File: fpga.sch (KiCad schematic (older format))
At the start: 107 parts, among them J14 JTAG, J19 TP_NORM_Y_G, J20 TP_RGB_COMP_X, J21 TP_HD_SD_X, SW1 FORCE_VIDEO, SW2 FORCE_VIDEO, U10 74LVC541A, U12 TC7SZ125FU, U15 10M08SC, U19 74LVC2G34, U5 74LVC14A, U6 74LVC14A, U7 74LVC14A, U9 KC2520Z50

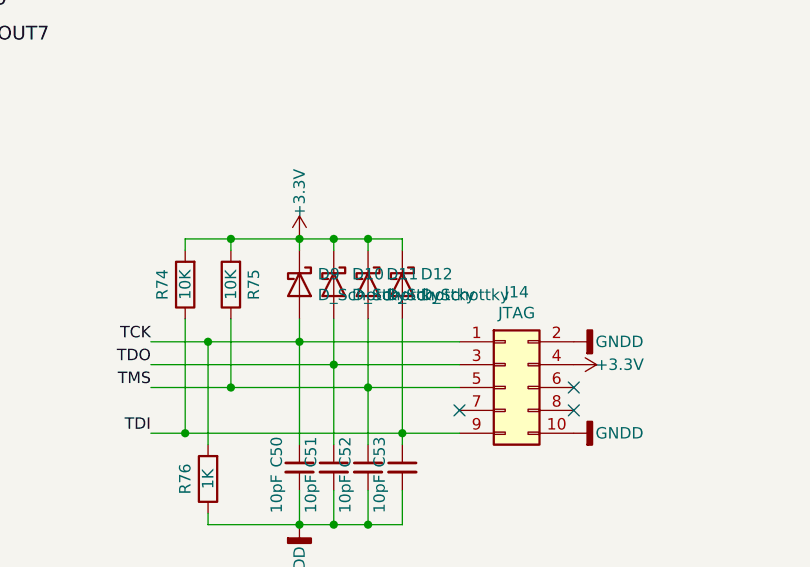
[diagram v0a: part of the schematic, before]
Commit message: Rev. E1
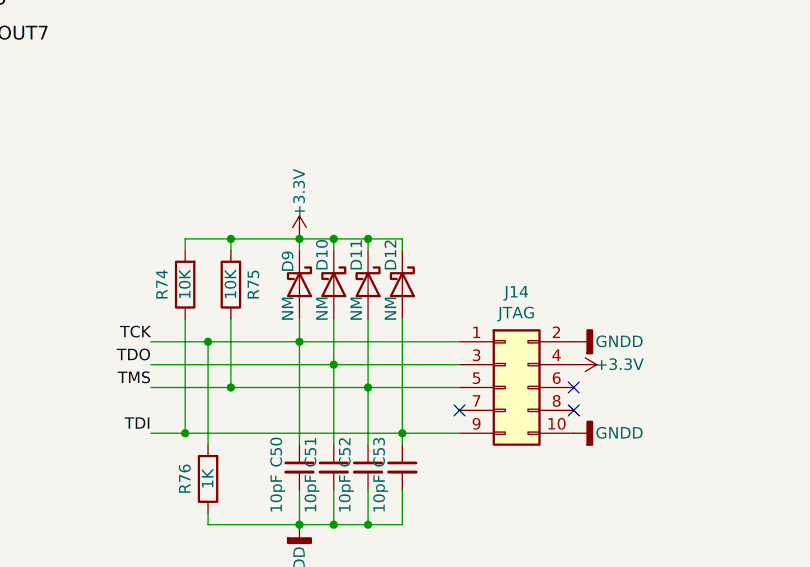
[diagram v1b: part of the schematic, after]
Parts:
- D10, D11, D12, D9: value D_Schottky -> NM
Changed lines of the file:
@@
 U 1 1 60BEE0A2
 P 8000 9450
-F 0 "D9" V 7954 9530 50  0000 L CNN
-F 1 "D_Schottky" V 8045 9530 50  0000 L CNN
+F 0 "D9" H 7850 9400 50  0000 L CNN
+F 1 "NM" H 8050 9400 50  0000 L CNN
 F 2 "Diode_SMD:D_SOD-123" H 8000 9450 50  0001 C CNN
 F 3 "~" H 8000 9450 50  0001 C CNN
@@
 U 1 1 60BFCE92
 P 8150 9450
-F 0 "D10" V 8104 9530 50  0000 L CNN
-F 1 "D_Schottky" V 8195 9530 50  0000 L CNN
+F 0 "D10" H 7950 9400 50  0000 L CNN
+F 1 "NM" H 8200 9400 50  0000 L CNN
 F 2 "Diode_SMD:D_SOD-123" H 8150 9450 50  0001 C CNN
 F 3 "~" H 8150 9450 50  0001 C CNN
@@
 U 1 1 60BFDBA6
 P 8300 9450
-F 0 "D11" V 8254 9530 50  0000 L CNN
-F 1 "D_Schottky" V 8345 9530 50  0000 L CNN
+F 0 "D11" H 8100 9400 50  0000 L CNN
+F 1 "NM" H 8350 9400 50  0000 L CNN
 F 2 "Diode_SMD:D_SOD-123" H 8300 9450 50  0001 C CNN
 F 3 "~" H 8300 9450 50  0001 C CNN
@@
 U 1 1 60BFE268
 P 8450 9450
-F 0 "D12" V 8404 9530 50  0000 L CNN
-F 1 "D_Schottky" V 8495 9530 50  0000 L CNN
+F 0 "D12" H 8250 9400 50  0000 L CNN
+F 1 "NM" H 8500 9400 50  0000 L CNN
 F 2 "Diode_SMD:D_SOD-123" H 8450 9450 50  0001 C CNN
 F 3 "~" H 8450 9450 50  0001 C CNN
